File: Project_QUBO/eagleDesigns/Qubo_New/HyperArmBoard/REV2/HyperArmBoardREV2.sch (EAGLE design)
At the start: 16 parts, among them U1 BME280

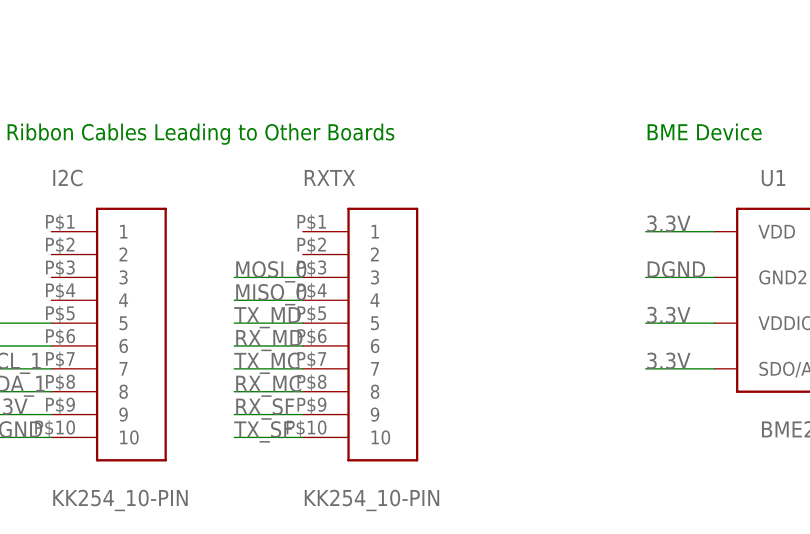
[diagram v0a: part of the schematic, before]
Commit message: changes to hyperarm and power board
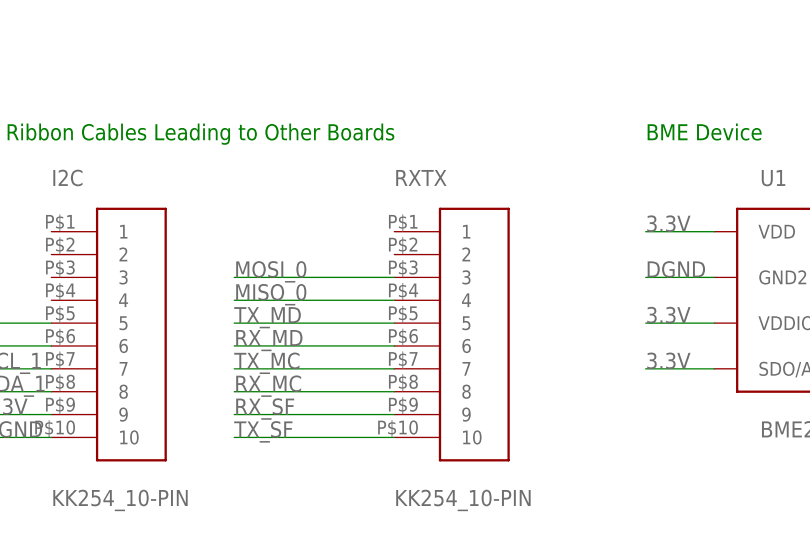
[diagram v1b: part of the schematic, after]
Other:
- moved on the sheet: RXTX
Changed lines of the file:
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@@
 <attribute name="NAME" x="48.26" y="152.4" size="1.778" layer="95"/>
 </instance>
-<instance part="RXTX" gate="G$1" x="167.64" y="33.02" smashed="yes">
-<attribute name="NAME" x="160.02" y="48.26" size="1.778" layer="95"/>
-<attribute name="VALUE" x="160.02" y="12.7" size="1.778" layer="96"/>
+<instance part="RXTX" gate="G$1" x="177.8" y="33.02" smashed="yes">
+<attribute name="NAME" x="170.18" y="48.26" size="1.778" layer="95"/>
+<attribute name="VALUE" x="170.18" y="12.7" size="1.778" layer="96"/>
 </instance>
 </instances>
@@
 <segment>
 <pinref part="RXTX" gate="G$1" pin="8"/>
-<wire x1="160.02" y1="25.4" x2="152.4" y2="25.4" width="0.1524" layer="91"/>
+<wire x1="170.18" y1="25.4" x2="152.4" y2="25.4" width="0.1524" layer="91"/>
 <label x="152.4" y="25.4" size="1.778" layer="95"/>
 </segment>
@@
 <segment>
 <pinref part="RXTX" gate="G$1" pin="7"/>
-<wire x1="160.02" y1="27.94" x2="152.4" y2="27.94" width="0.1524" layer="91"/>
+<wire x1="170.18" y1="27.94" x2="152.4" y2="27.94" width="0.1524" layer="91"/>
 <label x="152.4" y="27.94" size="1.778" layer="95"/>
 </segment>
@@
 <segment>
 <pinref part="RXTX" gate="G$1" pin="9"/>
-<wire x1="160.02" y1="22.86" x2="152.4" y2="22.86" width="0.1524" layer="91"/>
+<wire x1="170.18" y1="22.86" x2="152.4" y2="22.86" width="0.1524" layer="91"/>
 <label x="152.4" y="22.86" size="1.778" layer="95"/>
 </segment>
@@
 <segment>
 <pinref part="RXTX" gate="G$1" pin="10"/>
-<wire x1="160.02" y1="20.32" x2="152.4" y2="20.32" width="0.1524" layer="91"/>
+<wire x1="170.18" y1="20.32" x2="152.4" y2="20.32" width="0.1524" layer="91"/>
 <label x="152.4" y="20.32" size="1.778" layer="95"/>
 </segment>
@@
 <segment>
 <pinref part="RXTX" gate="G$1" pin="6"/>
-<wire x1="160.02" y1="30.48" x2="152.4" y2="30.48" width="0.1524" layer="91"/>
+<wire x1="170.18" y1="30.48" x2="152.4" y2="30.48" width="0.1524" layer="91"/>
 <label x="152.4" y="30.48" size="1.778" layer="95"/>
 </segment>
@@
 <segment>
 <pinref part="RXTX" gate="G$1" pin="5"/>
-<wire x1="160.02" y1="33.02" x2="152.4" y2="33.02" width="0.1524" layer="91"/>
+<wire x1="170.18" y1="33.02" x2="152.4" y2="33.02" width="0.1524" layer="91"/>
 <label x="152.4" y="33.02" size="1.778" layer="95"/>
 </segment>
@@
 <segment>
 <pinref part="RXTX" gate="G$1" pin="4"/>
-<wire x1="160.02" y1="35.56" x2="152.4" y2="35.56" width="0.1524" layer="91"/>
+<wire x1="170.18" y1="35.56" x2="152.4" y2="35.56" width="0.1524" layer="91"/>
 <label x="152.4" y="35.56" size="1.778" layer="95"/>
 </segment>
@@
 <segment>
 <pinref part="RXTX" gate="G$1" pin="3"/>
-<wire x1="160.02" y1="38.1" x2="152.4" y2="38.1" width="0.1524" layer="91"/>
+<wire x1="170.18" y1="38.1" x2="152.4" y2="38.1" width="0.1524" layer="91"/>
 <label x="152.4" y="38.1" size="1.778" layer="95"/>
 </segment>
